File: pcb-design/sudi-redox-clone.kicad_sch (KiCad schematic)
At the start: 113 parts, among them J1 RJ12_LEFT, J2 0.91 OLED, J3 RJ12_RIGHT, J5 USB_C, J7 ARMJTAG, J8 BatCon, K1 KEYSW, K10 KEYSW, K11 KEYSW, K12 KEYSW, K13 KEYSW, K14 KEYSW, K15 KEYSW, K16 KEYSW, K17 KEYSW, K18 KEYSW, K2 KEYSW, K3 KEYSW, K4 KEYSW, K5 KEYSW, K6 KEYSW, K7 KEYSW, K8 KEYSW, K9 KEYSW, SW1 RST, U4 AMS1117-3.3, U5 nRF51x22-QFxx, U6 TP4056, U8 MCP23017_SS, Y2 16MHz

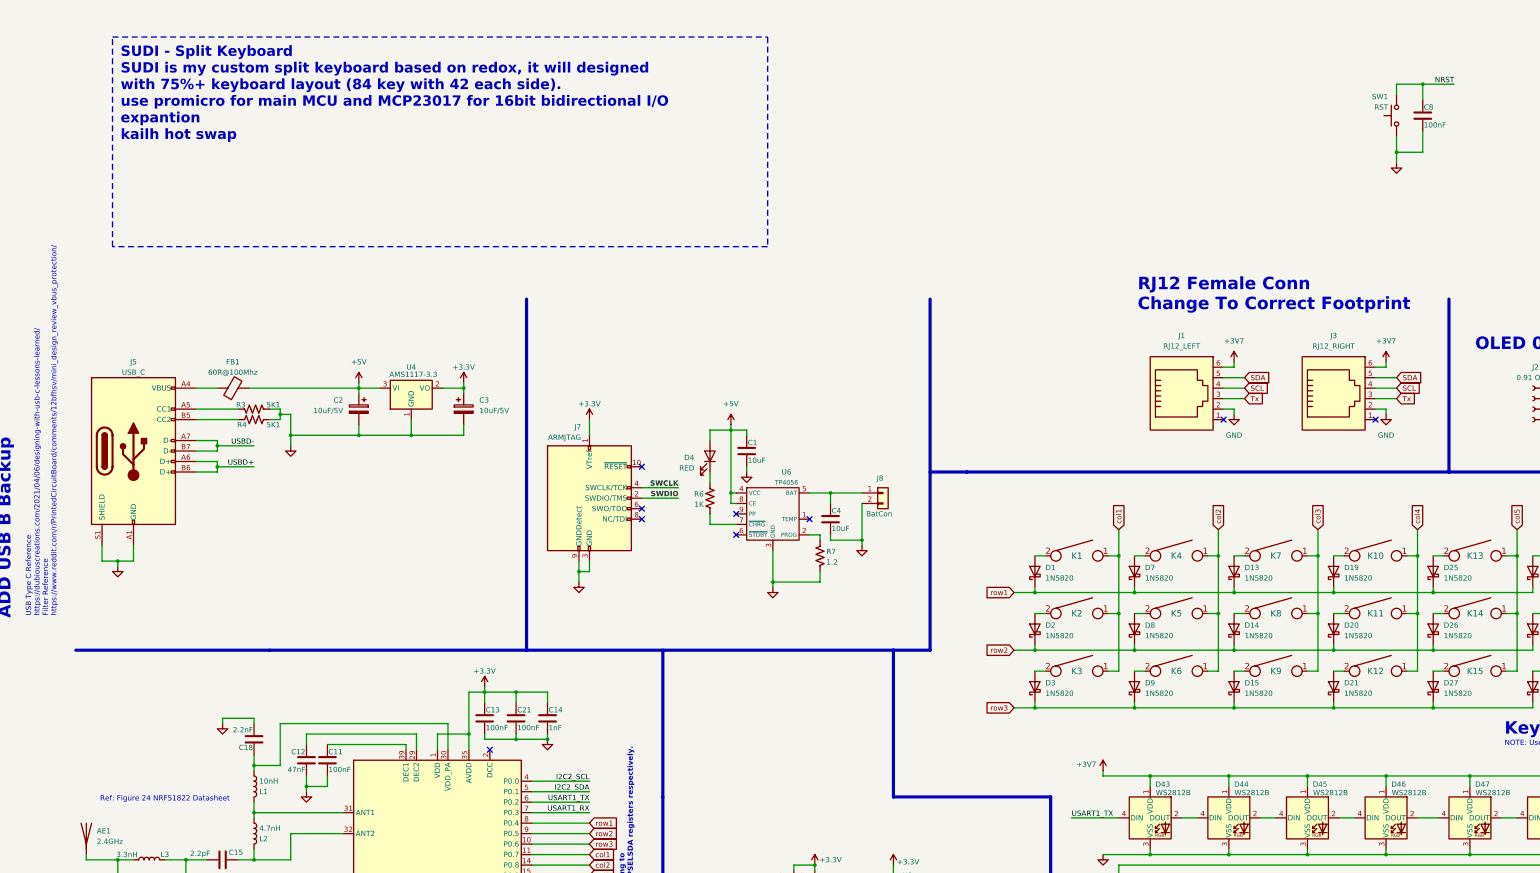
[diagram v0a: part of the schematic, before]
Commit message: [minggu 7 juli 12:12] create pcb cut profile
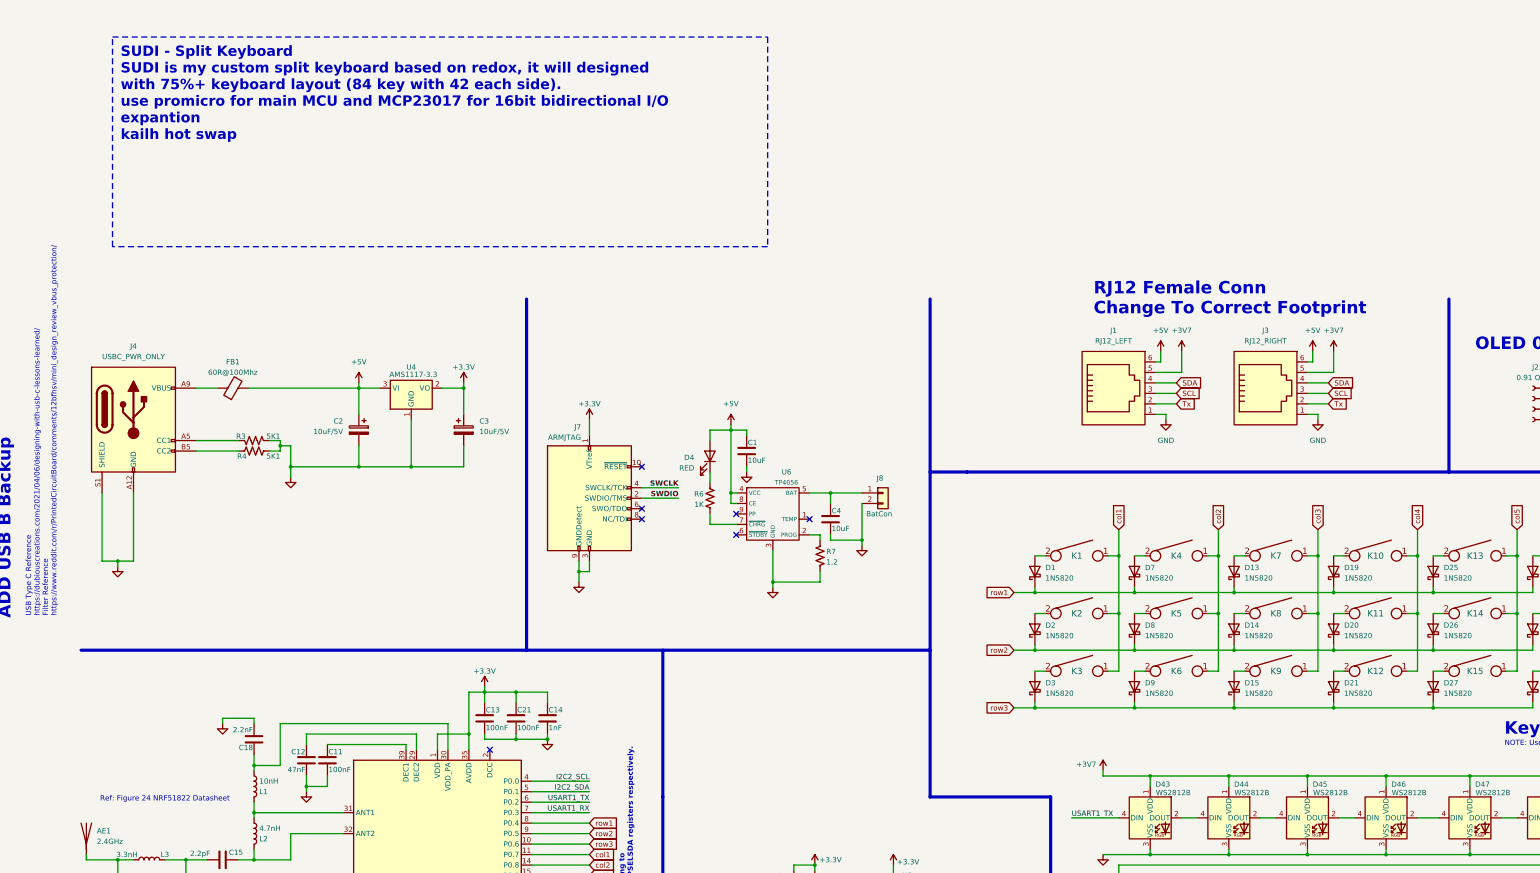
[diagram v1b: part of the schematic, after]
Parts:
- removed C8: 100nF, symbol Device:C
- removed J5: USB_C, symbol Connector:USB_C_Receptacle_USB2.0_14P
- removed SW1: RST, symbol Switch:SW_Push
- added J4: USBC_PWR_ONLY, Connector_USB:USB_C_Receptacle_GCT_USB4125-xx-x-0190_6P_TopMnt_Horizontal, symbol Connector:USB_C_Receptacle_PowerOnly_6P
- C1, C11, C12, C13, C14, C15, C16, C17, C18, C19, C2, C20, C21, C3, C4: footprint (none) -> Capacitor_SMD:C_0805_2012Metric_Pad1.18x1.45mm_HandSolder
- FB1, L1, L2, L3: footprint (none) -> Inductor_SMD:L_0603_1608Metric_Pad1.05x0.95mm_HandSolder
- J1, J3: footprint Connector_RJ:RJ12_Amphenol_54601 -> Connector_RJ:RJ25_Wayconn_MJEA-660X1_Horizontal
- J2: footprint KiCad-SSD1306-0.91-OLED-4pin-128x32:SSD1306-0.91-OLED-4pin-128x32 -> Connector_PinHeader_2.54mm:PinHeader_1x04_P2.54mm_Vertical
- J7: footprint (none) -> Connector_PinHeader_2.54mm:PinHeader_2x05_P2.54mm_Horizontal
- K2, K3: footprint canadian_footprints:Mx_Alps_150-dualsided -> canadian_footprints:Mx_Alps_100-dualside
- Y2: footprint (none) -> Crystal:Crystal_HC50_Vertical
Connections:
- net +3V7: now also J1.5, J3.5; no longer J1.6, J3.6
- net +5V: now also J1.6, J3.6
- net GND: now also J1.1, J3.1, J4.A12 (GND), J4.B12 (GND), J4.S1 (SHIELD); no longer J1.2, J3.2
- net SCL: now also J1.3, J3.3; no longer J1.4, J3.4
- net SDA: now also J1.4, J3.4; no longer J1.5, J3.5
- net Tx: now also J1.2, J3.2; no longer J1.3, J3.3
- net at R3.1: now also J4.A5 (CC1)
- net at R4.1: now also J4.B5 (CC2)
- net at FB1.1: now also J4.A9 (VBUS), J4.B9 (VBUS)
- no-connect marks 25 -> 23
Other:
- moved on the sheet: C2, C3, J1, R3, R4
